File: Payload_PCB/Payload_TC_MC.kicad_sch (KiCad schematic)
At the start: 8 parts, among them U3 MCP9601-E/MX

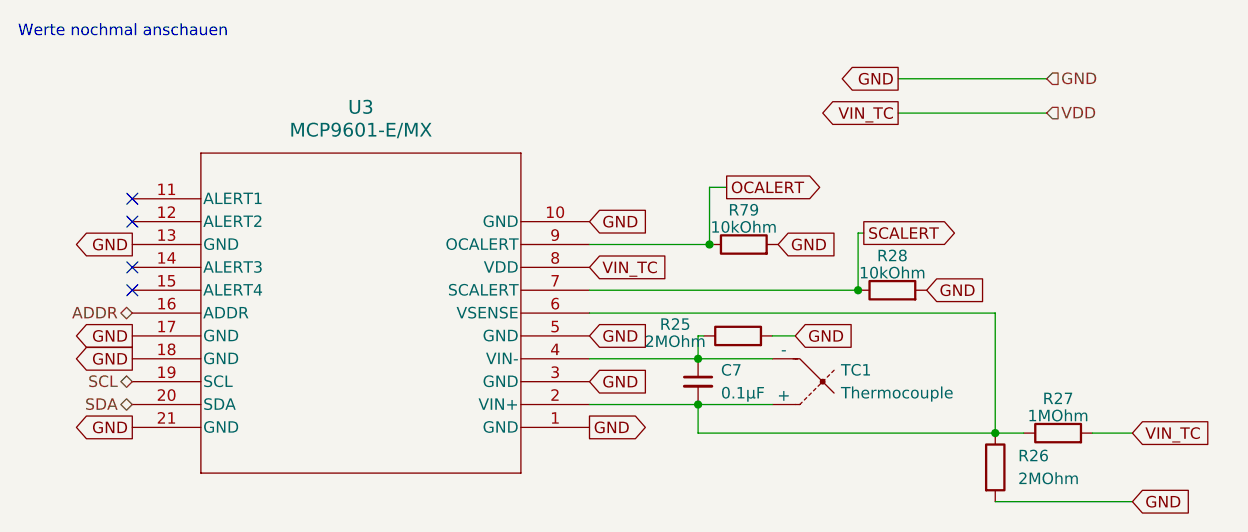
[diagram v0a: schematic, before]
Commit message: first parts layout
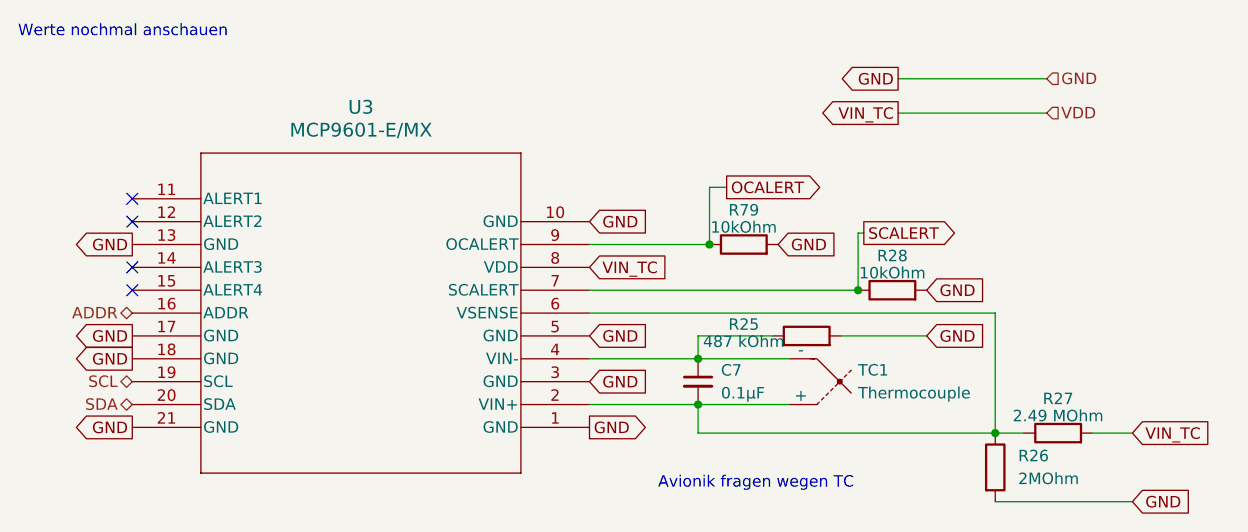
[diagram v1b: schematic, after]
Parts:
- R25: value 2MOhm -> 487 kOhm
- R27: value 1MOhm -> 2.49 MOhm
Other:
- note added: "Avionik fragen wegen TC"
- moved on the sheet: R25, TC1
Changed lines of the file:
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@@
     (stroke (width 0) (type default))
   )
-  (wire (pts (xy 116.84 78.74) (xy 125.095 78.74))
+  (wire (pts (xy 116.84 78.74) (xy 127 78.74))
     (stroke (width 0) (type default))
   )
@@
     (stroke (width 0) (type default))
   )
-  (wire (pts (xy 116.84 73.66) (xy 125.095 73.66))
+  (wire (pts (xy 116.84 73.66) (xy 127 73.66))
     (stroke (width 0) (type default))
   )
@@
     (stroke (width 0) (type default))
   )
-  (wire (pts (xy 125.095 71.12) (xy 127.635 71.12))
-    (stroke (width 0) (type default))
-  )
-  (wire (pts (xy 117.475 71.12) (xy 116.84 71.12))
+  (wire (pts (xy 132.715 71.12) (xy 142.24 71.12))
+    (stroke (width 0) (type default))
+  )
+  (wire (pts (xy 125.095 71.12) (xy 116.84 71.12))
     (stroke (width 0) (type default))
   )
@@
   (wire (pts (xy 139.065 46.355) (xy 155.575 46.355))
     (stroke (width 0) (type default))
+  )
+  (text "Avionik fragen wegen TC" (at 112.395 88.265 0)
+    (effects (font (size 1.27 1.27)) (justify left bottom))
   )
   (text "Werte nochmal anschauen" (at 41.275 38.1 0)
@@
     )
   )
-  (global_label "GND" (shape input) (at 127.635 71.12 0) (fields_autoplaced)
-    (effects (font (size 1.27 1.27)) (justify left))
-    (property "Intersheetrefs" "${INTERSHEET_REFS}" (at 134.4907 71.12 0)
+  (global_label "GND" (shape input) (at 142.24 71.12 0) (fields_autoplaced)
+    (effects (font (size 1.27 1.27)) (justify left))
+    (property "Intersheetrefs" "${INTERSHEET_REFS}" (at 149.0957 71.12 0)
       (effects (font (size 1.27 1.27)) (justify left) hide)
     )
@@
       (effects (font (size 1.27 1.27)))
     )
-    (property "Value" "1MOhm" (at 156.845 80.01 90)
+    (property "Value" "2.49 MOhm" (at 156.845 80.01 90)
       (effects (font (size 1.27 1.27)))
     )
@@
     )
   )
-  (symbol (lib_id "Device:Thermocouple") (at 127.635 76.2 180) (unit 1)
+  (symbol (lib_id "Device:Thermocouple") (at 129.54 76.2 180) (unit 1)
     (in_bom yes) (on_board yes) (dnp no) (fields_autoplaced)
-    (property "Reference" "TC1" (at 132.715 74.93 0)
+    (property "Reference" "TC1" (at 134.62 74.93 0)
       (effects (font (size 1.27 1.27)) (justify right))
     )
-    (property "Value" "Thermocouple" (at 132.715 77.47 0)
+    (property "Value" "Thermocouple" (at 134.62 77.47 0)
       (effects (font (size 1.27 1.27)) (justify right))
     )
-    (property "Footprint" "" (at 142.24 77.47 0)
-      (effects (font (size 1.27 1.27)) hide)
-    )
-    (property "Datasheet" "~" (at 142.24 77.47 0)
+    (property "Footprint" "" (at 144.145 77.47 0)
+      (effects (font (size 1.27 1.27)) hide)
+    )
+    (property "Datasheet" "~" (at 144.145 77.47 0)
       (effects (font (size 1.27 1.27)) hide)
     )
@@
     )
   )
-  (symbol (lib_id "Device:R") (at 121.285 71.12 90) (unit 1)
+  (symbol (lib_id "Device:R") (at 128.905 71.12 90) (unit 1)
     (in_bom yes) (on_board yes) (dnp no)
-    (property "Reference" "R25" (at 114.3 69.85 90)
-      (effects (font (size 1.27 1.27)))
-    )
-    (property "Value" "2MOhm" (at 114.3 71.755 90)
-      (effects (font (size 1.27 1.27)))
-    )
-    (property "Footprint" "" (at 121.285 72.898 90)
-      (effects (font (size 1.27 1.27)) hide)
-    )
-    (property "Datasheet" "~" (at 121.285 71.12 0)
-      (effects (font (size 1.27 1.27)) hide)
-    )
+    (property "Reference" "R25" (at 121.92 69.85 90)
+      (effects (font (size 1.27 1.27)))
+    )
+    (property "Value" "487 kOhm" (at 121.92 71.755 90)
+      (effects (font (size 1.27 1.27)))
+    )
+    (property "Footprint" "" (at 128.905 72.898 90)
+      (effects (font (size 1.27 1.27)) hide)
+    )
+    (property "Datasheet" "~" (at 128.905 71.12 0)
+      (effects (font (size 1.27 1.27)) hide)
+    )
